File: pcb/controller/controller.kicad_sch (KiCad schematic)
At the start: 17 parts, among them J1 USB_B, J2 ISP, J3 AudioJack3, J4 Conn_01x05, SW1 Function, SW2 Power, U1 ATtiny85-20P

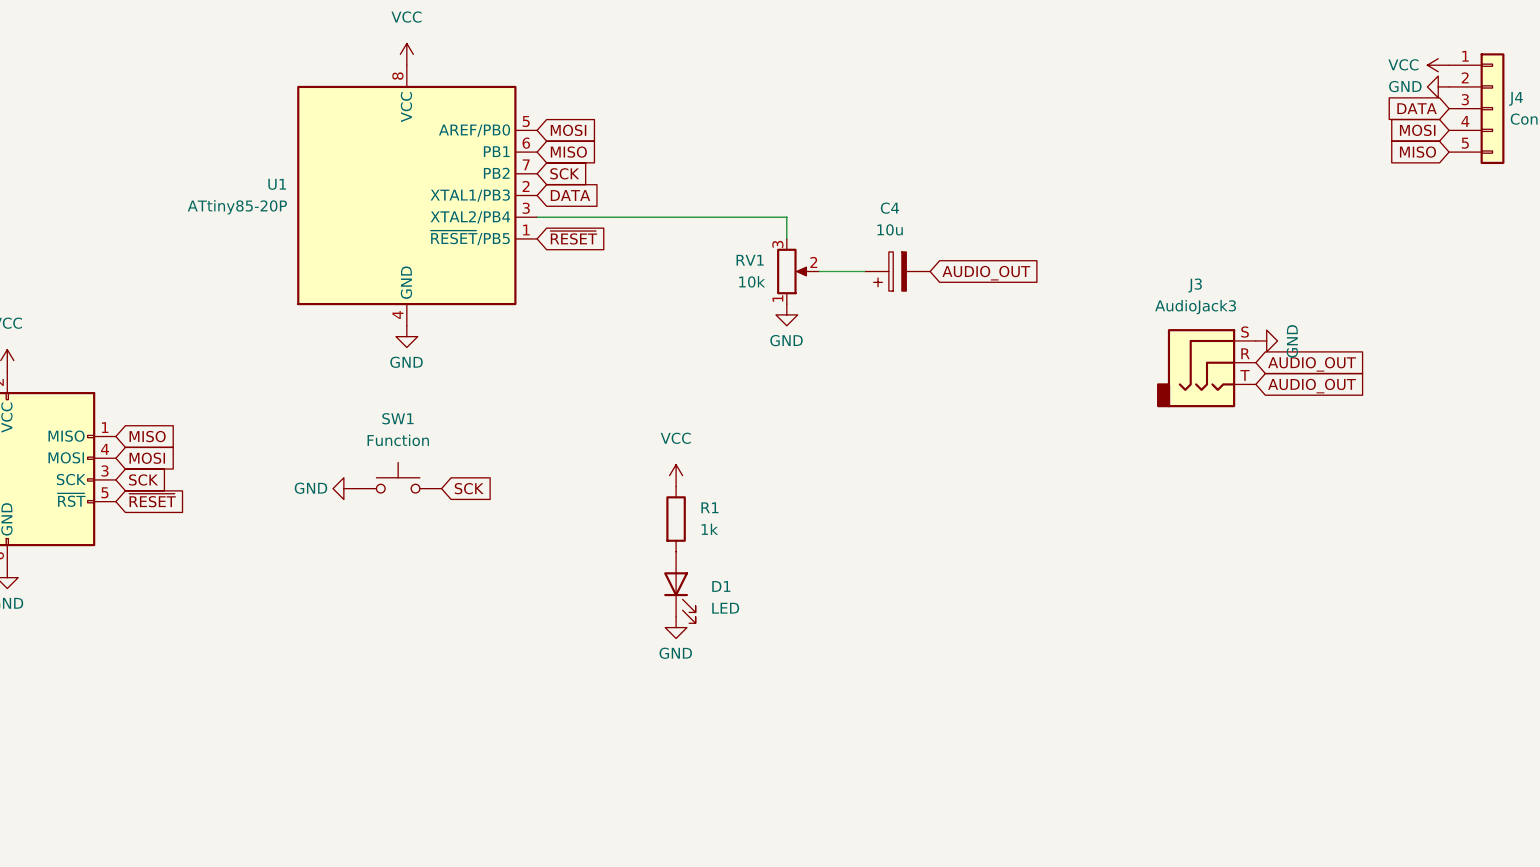
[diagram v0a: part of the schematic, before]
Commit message: Checkpoint
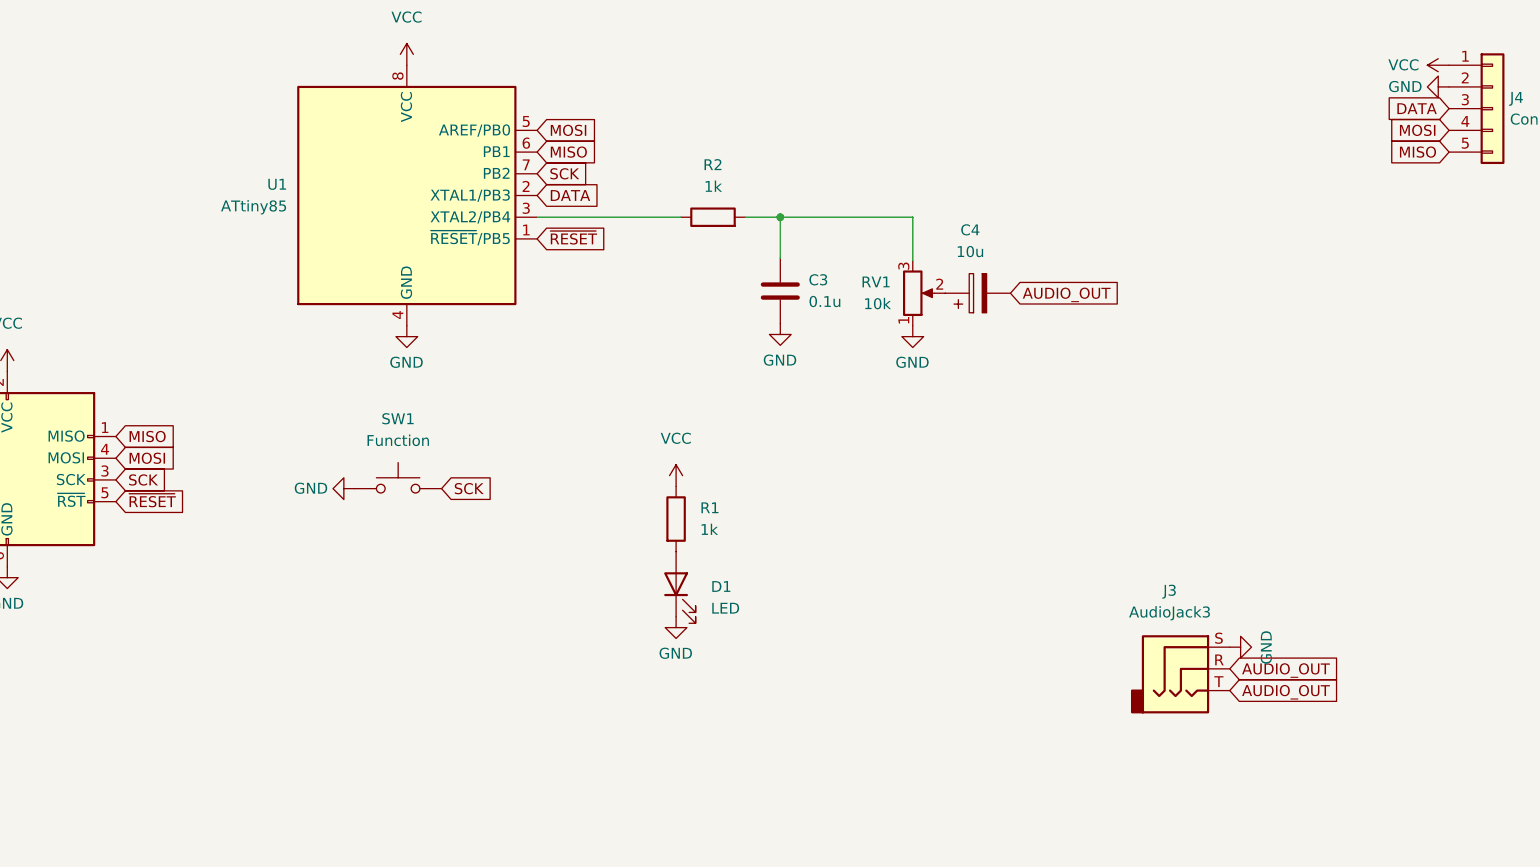
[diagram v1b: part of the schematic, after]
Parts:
- added C3: 0.1u, Capacitor_THT:C_Disc_D3.4mm_W2.1mm_P2.50mm, symbol Device:C
- added R2: 1k, Resistor_THT:R_Axial_DIN0207_L6.3mm_D2.5mm_P10.16mm_Horizontal, symbol Device:R
- J4: footprint Connector_PinHeader_2.54mm:PinHeader_1x05_P2.54mm_Horizontal -> Connector_PinHeader_2.54mm:PinHeader_1x05_P2.54mm_Vertical
- U1: value ATtiny85-20P -> ATtiny85
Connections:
- net GND: now also C3.2
- net at U1.3 (XTAL2/PB4): now also R2.1; no longer RV1.3
- new net: C3.1, R2.2, RV1.3
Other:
- moved on the sheet: C4, J3, RV1

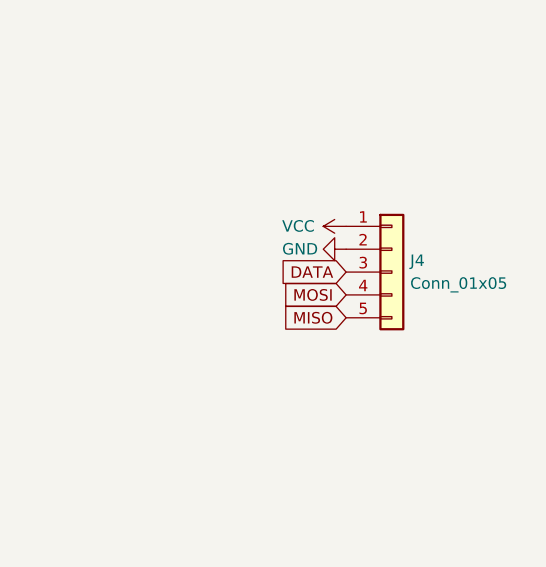
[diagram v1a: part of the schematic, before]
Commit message: Boards ordered.
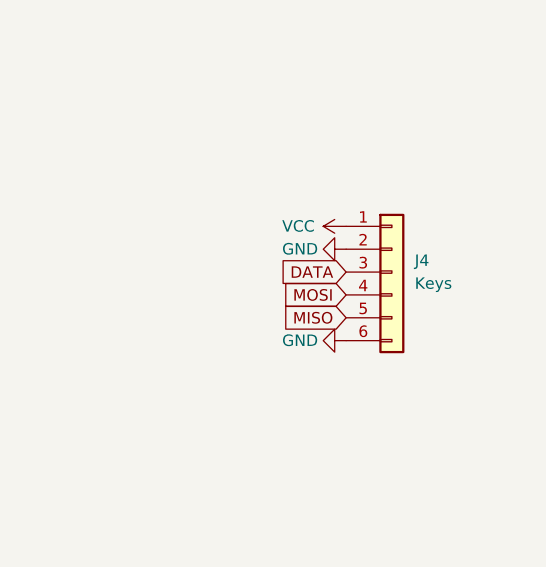
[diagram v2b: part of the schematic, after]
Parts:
- J4: value Conn_01x05 -> Keys; footprint Connector_PinHeader_2.54mm:PinHeader_1x05_P2.54mm_Vertical -> Connector_PinHeader_2.54mm:PinHeader_1x06_P2.54mm_Vertical; symbol Connector_Generic:Conn_01x05 -> Connector_Generic:Conn_01x06
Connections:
- net GND: now also J4.6 (Pin_6)
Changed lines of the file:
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@@
+    (pin "1")
+  )
+  (symbol (lib_id "power:GND") (at 219.71 74.676 270) (unit 1)
+    (in_bom yes) (on_board yes)
+    (property "Reference" "#PWR?" (id 0) (at 213.36 74.676 0)
+      (effects (font (size 1.27 1.27)) hide)
+    )
+    (property "Value" "GND" (id 1) (at 212.598 74.676 90)
+      (effects (font (size 1.27 1.27)) (justify left))
+    )
+    (property "Footprint" "" (id 2) (at 219.71 74.676 0)
+      (effects (font (size 1.27 1.27)) hide)
+    )
+    (property "Datasheet" "" (id 3) (at 219.71 74.676 0)
+      (effects (font (size 1.27 1.27)) hide)
+    )
     (pin "1")
   )
@@
     (pin "T")
   )
-  (symbol (lib_id "Connector_Generic:Conn_01x05") (at 224.79 67.056 0) (unit 1)
-    (in_bom yes) (on_board yes) (fields_autoplaced)
-    (property "Reference" "J4" (id 0) (at 226.822 65.7859 0)
-      (effects (font (size 1.27 1.27)) (justify left))
-    )
-    (property "Value" "Conn_01x05" (id 1) (at 226.822 68.3259 0)
-      (effects (font (size 1.27 1.27)) (justify left))
-    )
-    (property "Footprint" "Connector_PinHeader_2.54mm:PinHeader_1x05_P2.54mm_Vertical" (id 2) (at 224.79 67.056 0)
+  (symbol (lib_id "Connector_Generic:Conn_01x06") (at 224.79 67.056 0) (unit 1)
+    (in_bom yes) (on_board yes) (fields_autoplaced)
+    (property "Reference" "J4" (id 0) (at 227.33 65.7859 0)
+      (effects (font (size 1.27 1.27)) (justify left))
+    )
+    (property "Value" "Keys" (id 1) (at 227.33 68.3259 0)
+      (effects (font (size 1.27 1.27)) (justify left))
+    )
+    (property "Footprint" "Connector_PinHeader_2.54mm:PinHeader_1x06_P2.54mm_Vertical" (id 2) (at 224.79 67.056 0)
       (effects (font (size 1.27 1.27)) hide)
     )
@@
     (pin "4")
     (pin "5")
+    (pin "6")
   )
   (symbol (lib_id "power:VCC") (at 107.188 34.29 0) (unit 1)
@@
       (reference "#PWR0116") (unit 1) (value "GND") (footprint "")
     )
+    (path "/872e2402-ddd6-41ed-a42a-f5cc3ca2a255"
+      (reference "#PWR?") (unit 1) (value "GND") (footprint "")
+    )
     (path "/8ad58aaa-881f-4951-acc0-5fc27bce22e3"
       (reference "C1") (unit 1) (value "10u") (footprint "Capacitor_THT:CP_Radial_D5.0mm_P2.50mm")
@@
     )
     (path "/bf68bd7a-f204-47f8-973c-5fb899632703"
-      (reference "J4") (unit 1) (value "Conn_01x05") (footprint "Connector_PinHeader_2.54mm:PinHeader_1x05_P2.54mm_Vertical")
+      (reference "J4") (unit 1) (value "Keys") (footprint "Connector_PinHeader_2.54mm:PinHeader_1x06_P2.54mm_Vertical")
     )
     (path "/3a259560-8afb-487f-9ccd-4e59c4462820"

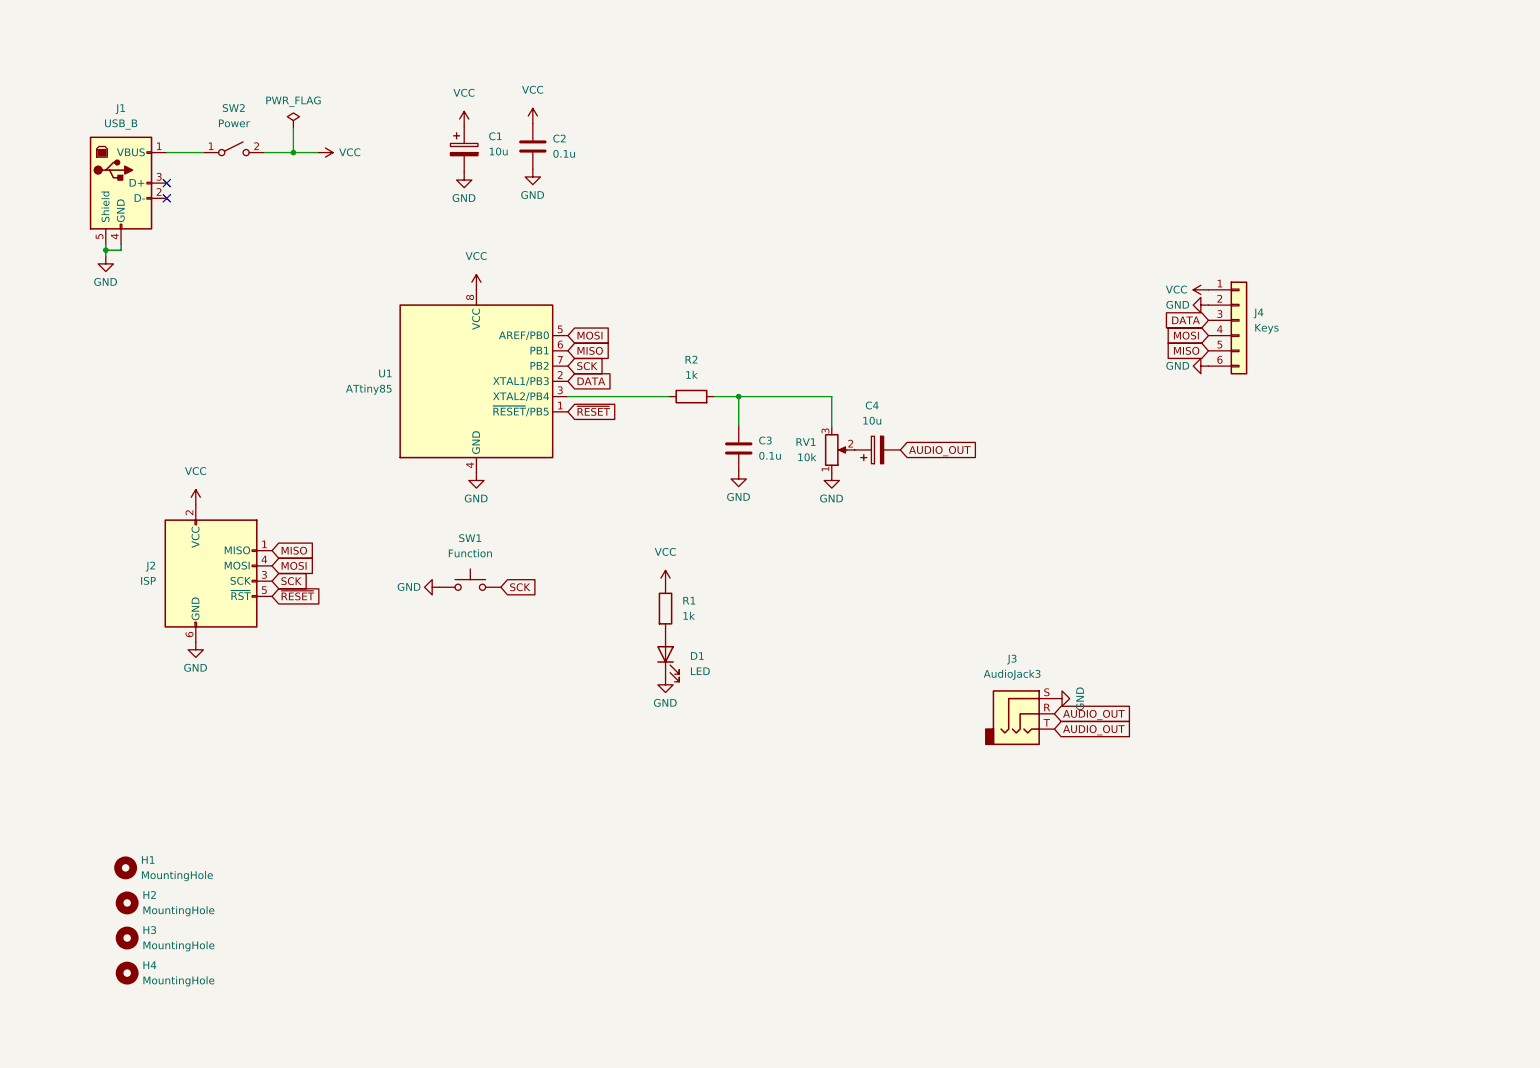
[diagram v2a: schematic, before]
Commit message: Checkpoint
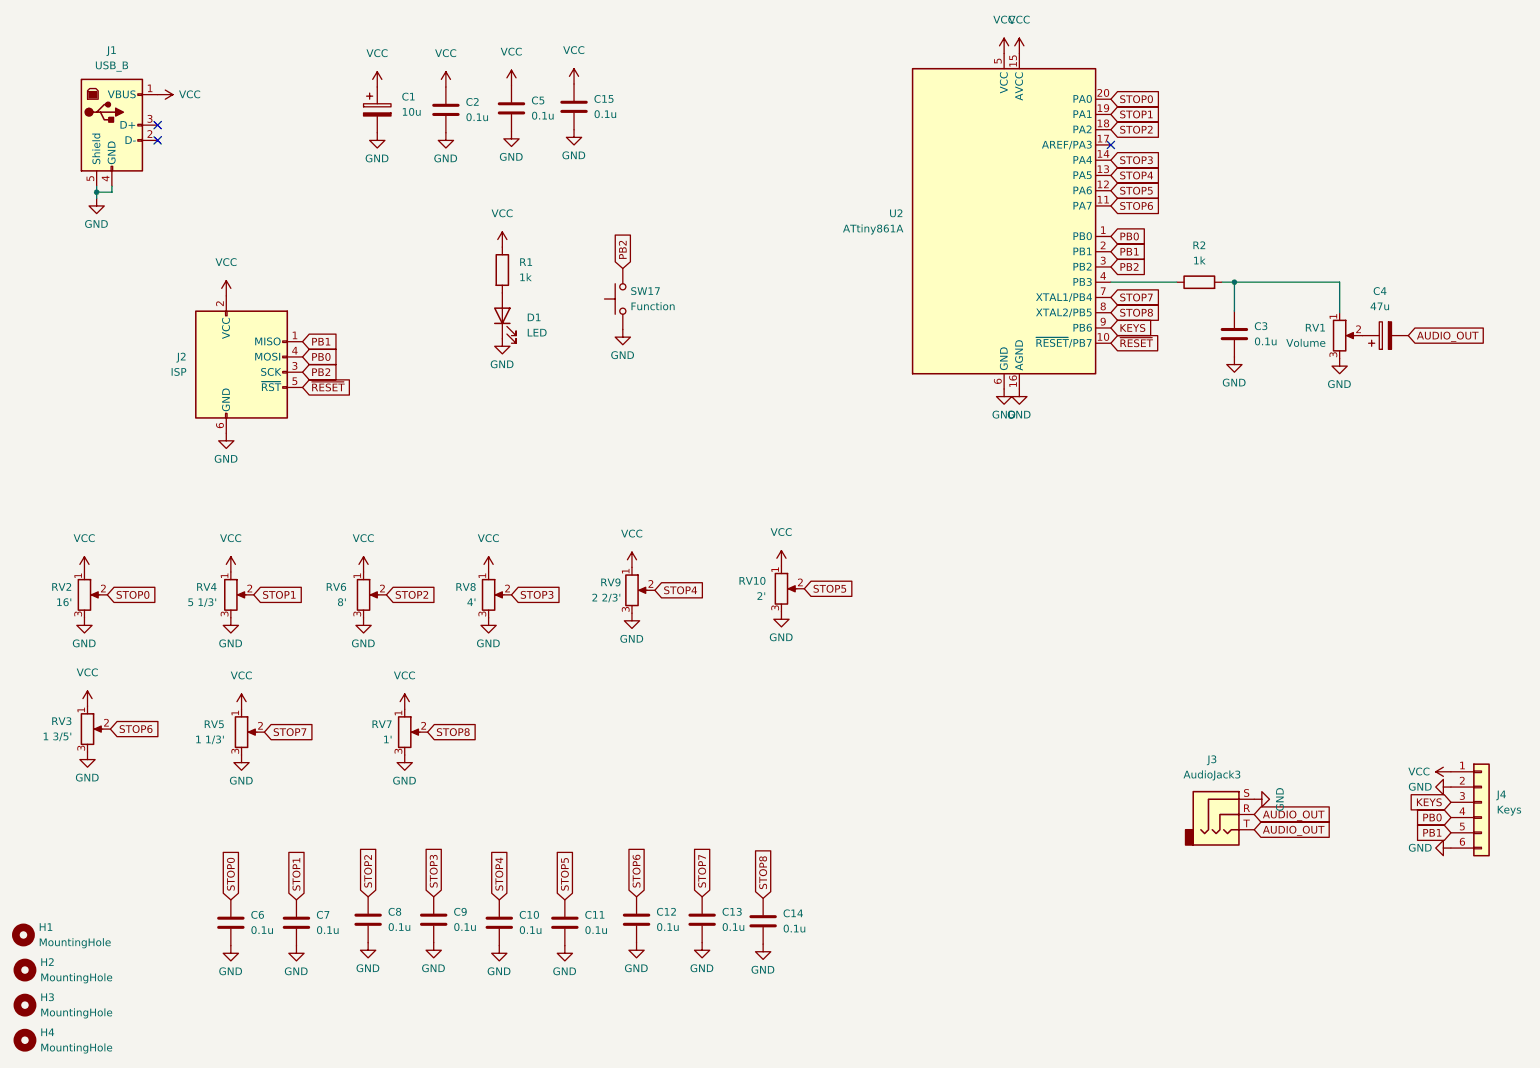
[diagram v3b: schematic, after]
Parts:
- removed SW1: Function, Button_Switch_THT:SW_PUSH_6mm, symbol Switch:SW_Push
- removed SW2: Power, Connector_PinHeader_2.54mm:PinHeader_1x03_P2.54mm_Vertical, symbol Switch:SW_SPST
- removed U1: ATtiny85, Package_DIP:DIP-8_W7.62mm, symbol MCU_Microchip_ATtiny:ATtiny85-20P
- added C10, C11, C12, C13, C14, C15, C5, C6, C7, C8, C9: 0.1u, Capacitor_THT:C_Disc_D3.0mm_W2.0mm_P2.50mm, symbol Device:C
- added RV10: 2', Potentiometer_THT:Potentiometer_Bourns_PTA3043_Single_Slide, symbol Device:R_Potentiometer
- added RV2: 16', Potentiometer_THT:Potentiometer_Bourns_PTA3043_Single_Slide, symbol Device:R_Potentiometer
- added RV3: 1 3/5', Potentiometer_THT:Potentiometer_Bourns_PTA3043_Single_Slide, symbol Device:R_Potentiometer
- added RV4: 5 1/3', Potentiometer_THT:Potentiometer_Bourns_PTA3043_Single_Slide, symbol Device:R_Potentiometer
- added RV5: 1 1/3', Potentiometer_THT:Potentiometer_Bourns_PTA3043_Single_Slide, symbol Device:R_Potentiometer
- added RV6: 8', Potentiometer_THT:Potentiometer_Bourns_PTA3043_Single_Slide, symbol Device:R_Potentiometer
- added RV7: 1', Potentiometer_THT:Potentiometer_Bourns_PTA3043_Single_Slide, symbol Device:R_Potentiometer
- added RV8: 4', Potentiometer_THT:Potentiometer_Bourns_PTA3043_Single_Slide, symbol Device:R_Potentiometer
- added RV9: 2 2/3', Potentiometer_THT:Potentiometer_Bourns_PTA3043_Single_Slide, symbol Device:R_Potentiometer
- added SW17: Function, Button_Switch_THT:SW_PUSH_6mm, symbol Switch:SW_Push
- added U2: ATtiny861A, Package_DIP:DIP-20_W7.62mm, symbol MCU_Microchip_ATtiny:ATtiny861A-P
- C1: footprint Capacitor_THT:CP_Radial_D5.0mm_P2.50mm -> Capacitor_THT:CP_Radial_D5.0mm_P2.00mm; LCSC (none) -> C15850
- C2, C3: footprint Capacitor_THT:C_Disc_D3.4mm_W2.1mm_P2.50mm -> Capacitor_THT:C_Disc_D3.0mm_W2.0mm_P2.50mm; LCSC (none) -> C49678
- C4: value 10u -> 47u; footprint Capacitor_THT:CP_Radial_D5.0mm_P2.50mm -> Capacitor_THT:CP_Radial_D5.0mm_P2.00mm; LCSC (none) -> C15850
- D1: LCSC (none) -> C2297
- R1, R2: footprint Resistor_THT:R_Axial_DIN0207_L6.3mm_D2.5mm_P10.16mm_Horizontal -> Resistor_THT:R_Axial_DIN0309_L9.0mm_D3.2mm_P15.24mm_Horizontal; LCSC (none) -> C17513
- RV1: value 10k -> Volume; footprint Potentiometer_THT:Potentiometer_Bourns_3386P_Vertical -> Potentiometer_THT:Potentiometer_Bourns_PTA3043_Single_Slide
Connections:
- net GND: now also RV1.3, C10.2, C11.2, C12.2, C13.2, C14.2, C15.2, C5.2, C6.2, C7.2, C8.2, C9.2, RV10.3, RV2.3, RV3.3, RV4.3, RV5.3, RV6.3, RV7.3, RV8.3, RV9.3, SW17.1, U2.16 (AGND), U2.6 (GND); no longer RV1.1
- net VCC: now also J1.1 (VBUS), C15.1, C5.1, RV10.1, RV2.1, RV3.1, RV4.1, RV5.1, RV6.1, RV7.1, RV8.1, RV9.1, U2.15 (AVCC), U2.5 (VCC)
- net ~{RESET}: now also U2.10 (~{RESET}/PB7)
- net at R2.1: now also U2.4 (PB3)
- net at C3.1, R2.2: now also RV1.1; no longer RV1.3
- net DATA renamed KEYS
- net KEYS: now also U2.9 (PB6)
- net MISO renamed PB1
- net PB1: now also U2.2 (PB1)
- net MOSI renamed PB0
- net PB0: now also U2.1 (PB0)
- net SCK renamed PB2
- net PB2: now also SW17.2, U2.3 (PB2)
- new net STOP0: C6.1, RV2.2, U2.20 (PA0)
- new net STOP1: C7.1, RV4.2, U2.19 (PA1)
- new net STOP2: C8.1, RV6.2, U2.18 (PA2)
- new net STOP3: C9.1, RV8.2, U2.14 (PA4)
- new net STOP4: C10.1, RV9.2, U2.13 (PA5)
- new net STOP5: C11.1, RV10.2, U2.12 (PA6)
- new net STOP6: C12.1, RV3.2, U2.11 (PA7)
- new net STOP7: C13.1, RV5.2, U2.7 (XTAL1/PB4)
- new net STOP8: C14.1, RV7.2, U2.8 (XTAL2/PB5)
- no-connect marks 2 -> 3
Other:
- moved on the sheet: C1, C2, C3, C4, D1, H1, H2, H3, H4, J1, J2, J3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
